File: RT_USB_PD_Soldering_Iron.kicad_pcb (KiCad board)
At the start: 4 copper layers, 75 x 11 mm, 63 parts, among them J1 USB4105-GF-A, J2 35RASMT4BHNTRX, SW1 SW_Push, SW2 SW_Push, U1 SPX3819M5-L-3-3, U2 BMI270, U3 DRTR5V0U4S-7, U5 STM32G431Kxxx, U6 TPS25982ONRGET, U7 OPA376AIDCKR, U8 STTS22H, Y1 NX2016SA-24MHZ-EXS00A-CS10820

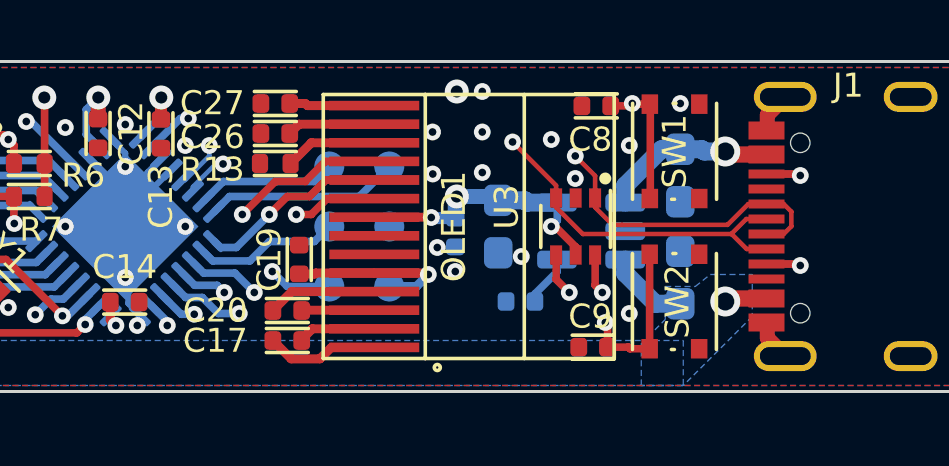
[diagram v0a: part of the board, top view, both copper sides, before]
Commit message: more usb improvements
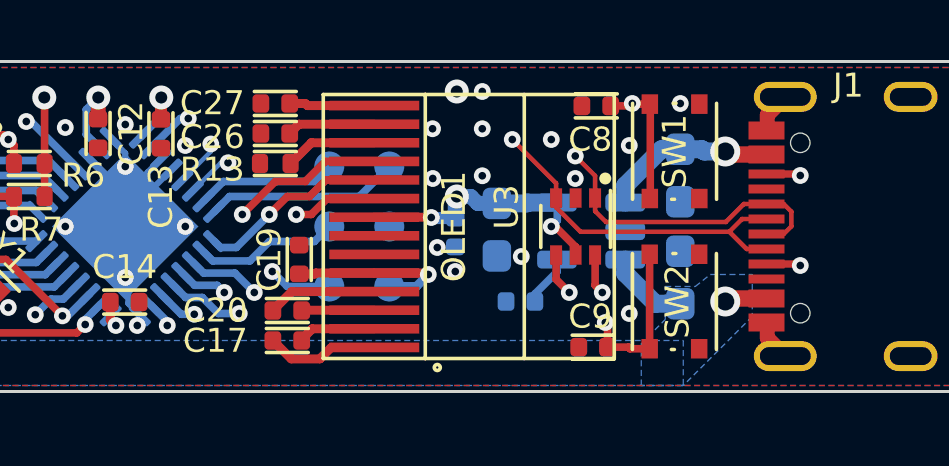
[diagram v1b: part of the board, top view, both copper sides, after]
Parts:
- moved C2 0.11 mm to (159.6, 125.1)
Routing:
- net /CC2: track 24.8 -> 25.9 mm
